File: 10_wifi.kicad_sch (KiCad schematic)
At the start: 24 parts, among them J24 Conn_01x04, J25 Conn_01x04, J26 TYPE-C-31-M-12, J27 Conn_01x03, J28 Conn_01x03, J29 EnUSB, U12 FC41D, U13 TLV62130

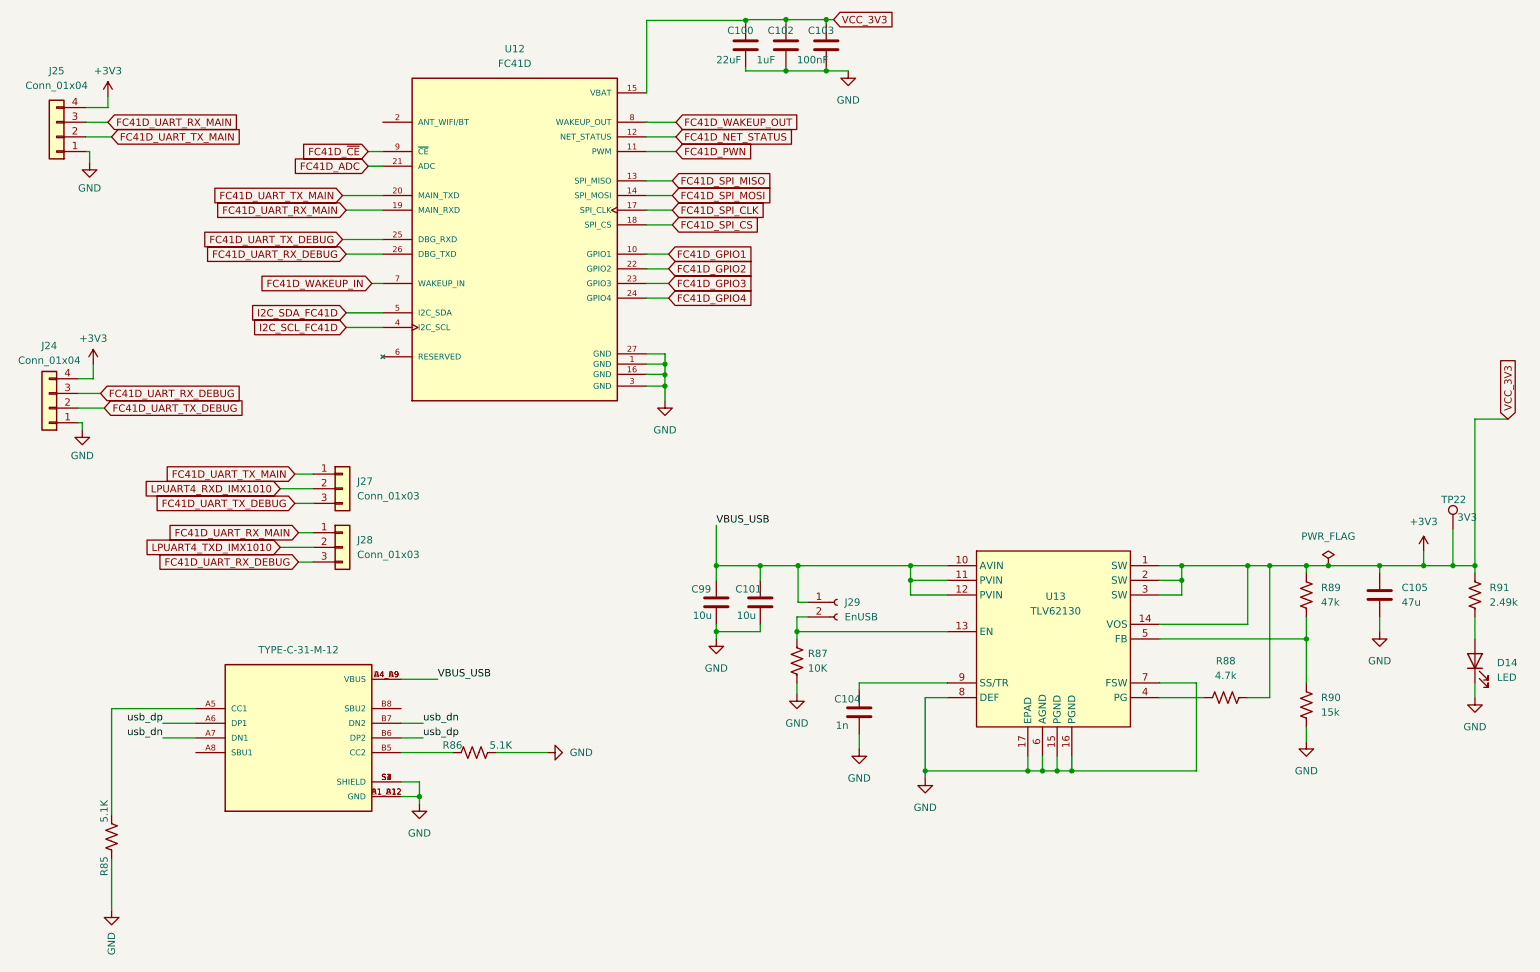
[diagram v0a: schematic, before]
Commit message: dad
da
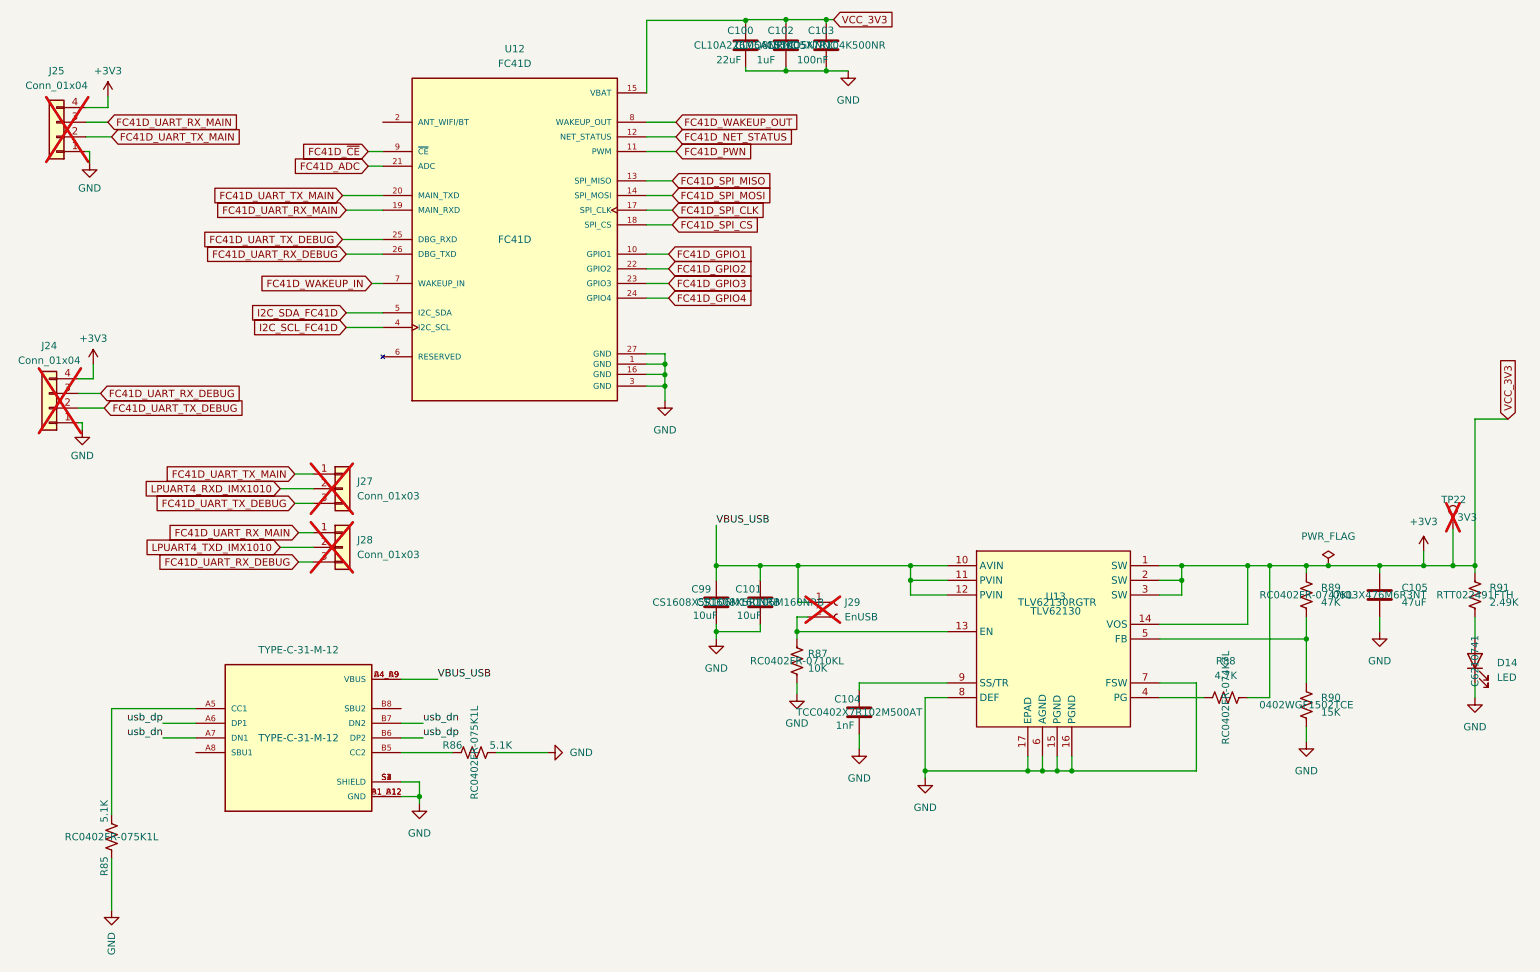
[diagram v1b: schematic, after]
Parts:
- C100: footprint Resistor_SMD:R_0603_1608Metric -> Capacitor_SMD:C_0603_1608Metric; Manufacturer_Part_Number (none) -> CL10A226MQ8NRNC
- C101, C99: value 10u -> 10uF; Manufacturer_Part_Number (none) -> CS1608X5R106M160NRB
- C102: Manufacturer_Part_Number (none) -> CL05A105KO5NNNC
- C103: Manufacturer_Part_Number (none) -> CS1005X7R104K500NR
- C104: value 1n -> 1nF; Manufacturer_Part_Number (none) -> TCC0402X7R102M500AT
- C105: value 47u -> 47uF; Manufacturer_Part_Number (none) -> 0603X476M6R3NT
- D14: Manufacturer_Part_Number (none) -> C6210741
- J24, J25, J27, J28, J29, TP22: now not fitted
- J26: Manufacturer_Part_Number (none) -> TYPE-C-31-M-12
- R85, R86: Manufacturer_Part_Number (none) -> RC0402FR-075K1L
- R87: Manufacturer_Part_Number (none) -> RC0402FR-0710KL
- R88: value 4.7k -> 4.7K; Manufacturer_Part_Number (none) -> RC0402FR-074K7L
- R89: value 47k -> 47K; Manufacturer_Part_Number (none) -> RC0402FR-0747KL
- R90: value 15k -> 15K; Manufacturer_Part_Number (none) -> 0402WGF1502TCE
- R91: value 2.49k -> 2.49K; Manufacturer_Part_Number (none) -> RTT022491FTH
- U12: Manufacturer_Part_Number (none) -> FC41D
- U13: Manufacturer_Part_Number (none) -> TLV62130RGTR

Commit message: gema
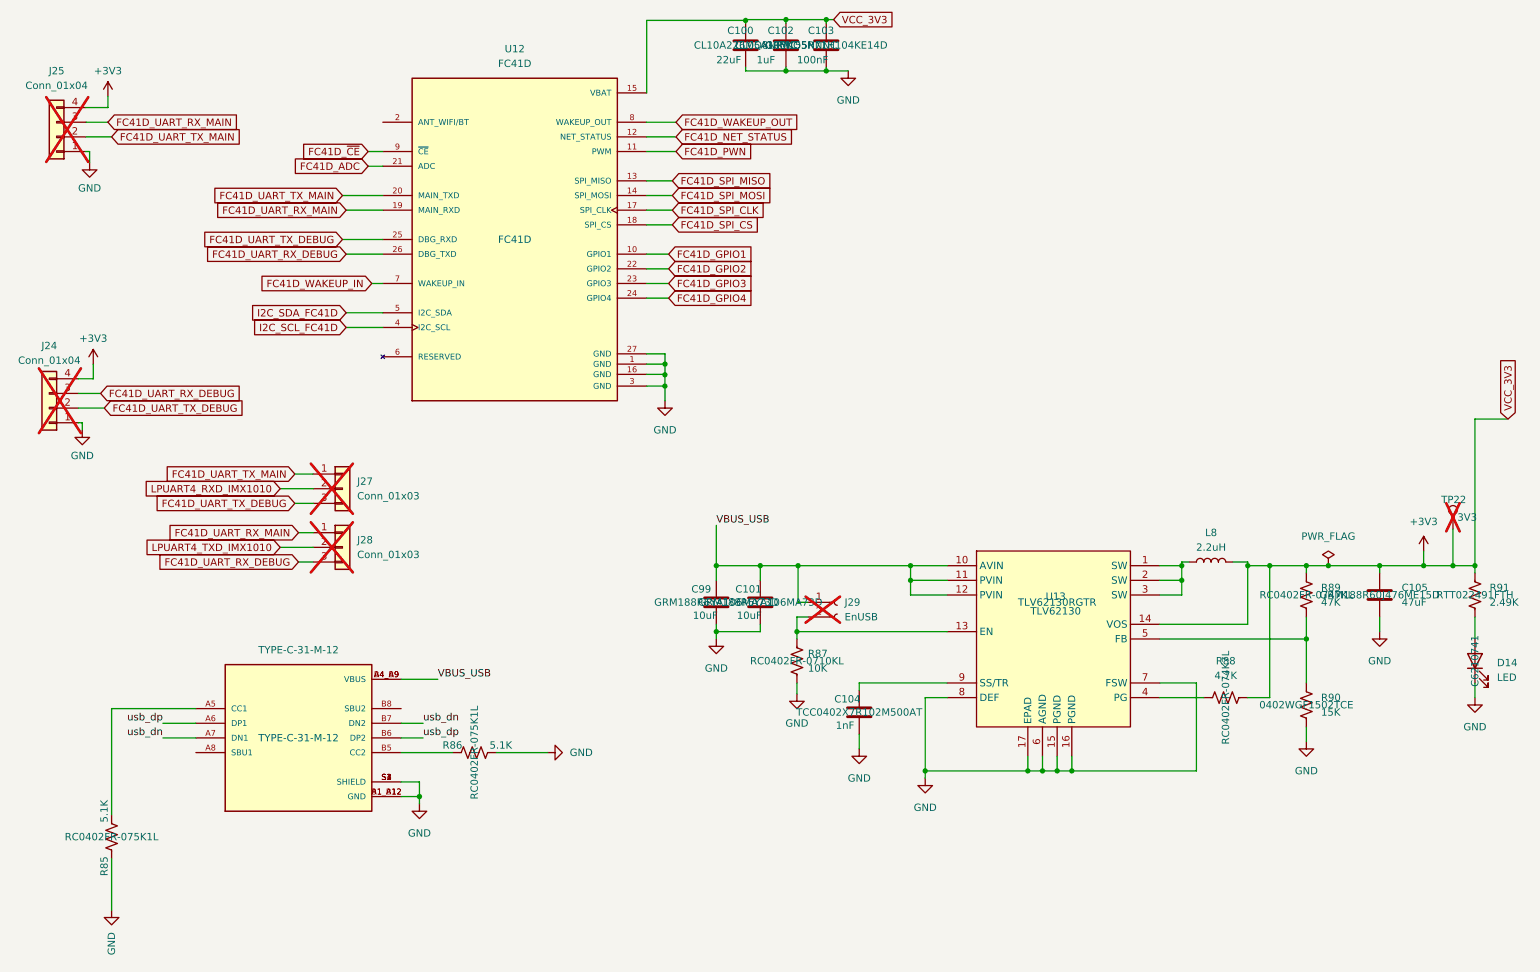
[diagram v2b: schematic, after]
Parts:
- added L8: 2.2uH, symbol Device:L
- C100:  LCSC Part # (none) -> C59461
- C101, C99:  LCSC Part # (none) -> C194427; Manufacturer_Part_Number CS1608X5R106M160NRB -> GRM188R6YA106MA73D
- C102:  LCSC Part # (none) -> C29266
- C103:  LCSC Part # (none) -> C77020; Manufacturer_Part_Number CS1005X7R104K500NR -> GRM155R71H104KE14D
- C104:  LCSC Part # (none) -> C696907
- C105:  LCSC Part # (none) -> C140782; Manufacturer_Part_Number 0603X476M6R3NT -> GRM188R60J476ME15D
- D14:  LCSC Part # (none) -> C6210741
- J26:  LCSC Part # (none) -> C165948
- R85, R86:  LCSC Part # (none) -> C105872
- R87:  LCSC Part # (none) -> C60490
- R88:  LCSC Part # (none) -> C105871
- R89:  LCSC Part # (none) -> C93943
- R90:  LCSC Part # (none) -> C25756
- R91:  LCSC Part # (none) -> C102924
- U12:  LCSC Part # (none) -> FC41D
- U13:  LCSC Part # (none) -> C122479
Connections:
- net +3V3: now also L8.2; no longer U13.1 (SW), U13.2 (SW), U13.3 (SW)
- new net: L8.1, U13.1 (SW), U13.2 (SW), U13.3 (SW)
